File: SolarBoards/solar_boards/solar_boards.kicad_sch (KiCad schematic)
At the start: 18 parts, among them J1 M55-6001242R, U1 TPS61089

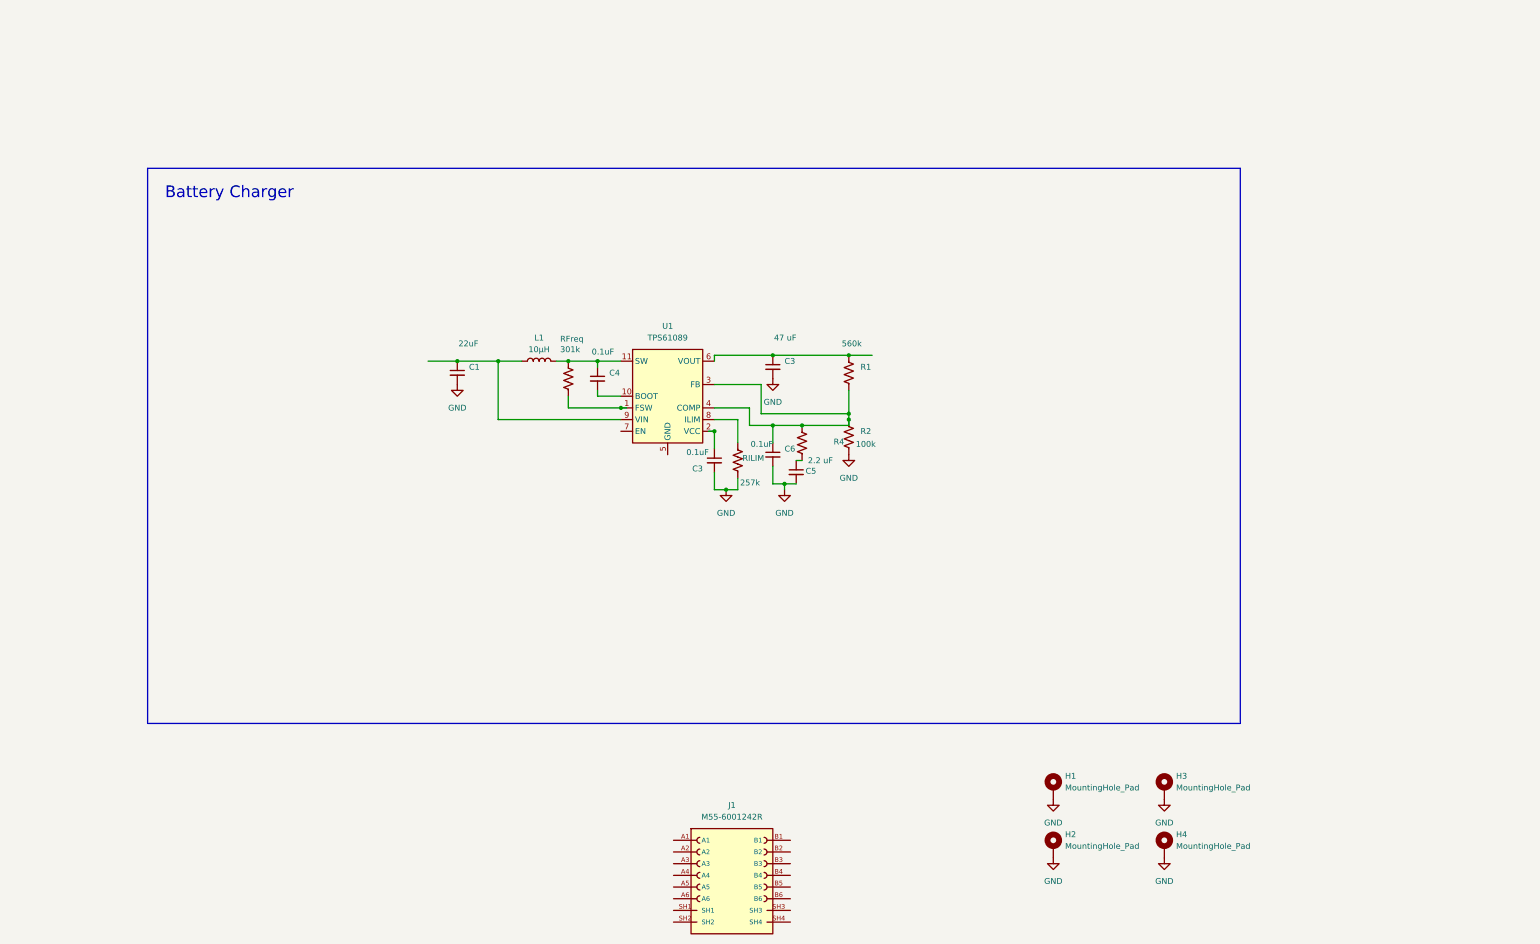
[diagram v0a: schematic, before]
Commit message: Solar Board Schematic and Routing
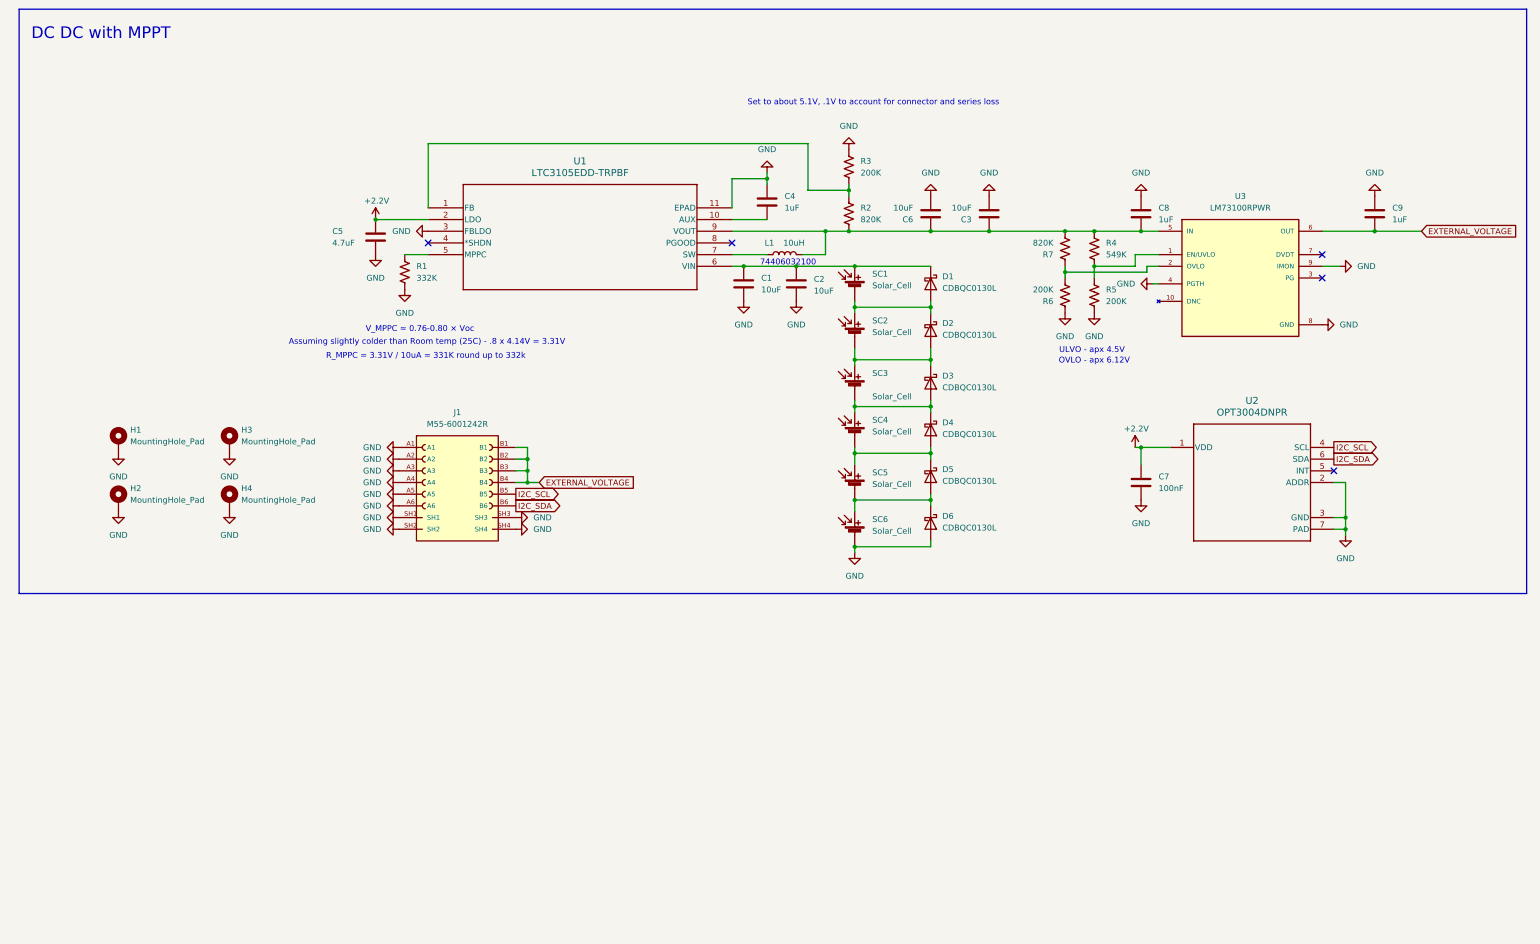
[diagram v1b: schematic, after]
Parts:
- removed C1: 22uF, symbol Device:C_Small
- removed C3: 47 uF, symbol Device:C_Small
- removed C3, C4, C6: 0.1uF, symbol Device:C_Small
- removed C5: 2.2 uF, symbol Device:C_Small
- removed RFreq: 301k, symbol Device:R_US
- removed RILIM: 257k, symbol Device:R_US
- removed U1: TPS61089, Package_DFN_QFN:Texas_VQFN-RNR0011A-11, symbol Regulator_Switching:TPS61089
- added C1, C2, C3, C6: 10uF, Capacitor_SMD:C_0402_1005Metric_Pad0.74x0.62mm_HandSolder, symbol Device:C
- added C4, C8, C9: 1uF, Capacitor_SMD:C_0402_1005Metric_Pad0.74x0.62mm_HandSolder, symbol Device:C
- added C5: 4.7uF, Capacitor_SMD:C_0402_1005Metric_Pad0.74x0.62mm_HandSolder, symbol Device:C
- added C7: 100nF, Capacitor_SMD:C_0402_1005Metric_Pad0.74x0.62mm_HandSolder, symbol Device:C
- added D1, D2, D3, D4, D5, D6: CDBQC0130L, inspireFly:DIODFN100X60X55-2N, symbol Device:D_Schottky
- added R3, R5, R6: 200K, Resistor_SMD:R_0402_1005Metric_Pad0.72x0.64mm_HandSolder, symbol Device:R_US
- added R7: 820K, Resistor_SMD:R_0402_1005Metric_Pad0.72x0.64mm_HandSolder, symbol Device:R_US
- added SC1, SC2, SC3, SC4, SC5, SC6: Solar_Cell, inspireFly:SOLAR_KXOB25-14X1F-TR, symbol Device:Solar_Cell
- added U1: LTC3105EDD-TRPBF, inspireFly:DFN-10_DD_LIT, symbol inspireFly:LTC3105EDD-TRPBF
- added U2: OPT3004DNPR, inspireFly:DNP0006A, symbol 2026-04-11_18-01-49:OPT3004DNPR
- added U3: LM73100RPWR, inspireFly:IC_LM73100RPWR, symbol inspireFly:LM73100RPWR
- L1: value 10µH -> 10uH; footprint (none) -> inspireFly:WE-LQFS_3818
- R1: value 560k -> 332K; footprint (none) -> Resistor_SMD:R_0402_1005Metric_Pad0.72x0.64mm_HandSolder
- R2: value 100k -> 820K; footprint (none) -> Resistor_SMD:R_0402_1005Metric_Pad0.72x0.64mm_HandSolder
- R4: value R_US -> 549K; footprint (none) -> Resistor_SMD:R_0402_1005Metric_Pad0.72x0.64mm_HandSolder
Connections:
- net GND: now also J1.A1, J1.A2, J1.A3, J1.A4, J1.A5, J1.A6, J1.SH1, J1.SH2, J1.SH3, J1.SH4, R1.2, C1.2, C2.2, C3.2, C4.1, C5.2, C6.2, C7.2, C8.2, C9.2, D6.2 (A), R3.1, R5.2, R6.1, SC6.2 (-), U1.11 (EPAD), U1.3 (FBLDO), U2.2 (ADDR), U2.3 (GND), U2.7 (PAD), U3.4 (PGTH), U3.8 (GND), U3.9 (IMON); no longer R2.2
- net at R4.2: now also R5.1, U3.1 (EN/UVLO)
- net at L1.1: now also U1.7 (SW)
- net at L1.2: now also R2.2, R4.1, C3.1, C6.1, C8.1, R7.2, U1.9 (VOUT), U3.5 (IN)
- net at R1.1: now also U1.5 (MPPC)
- net EXTERNAL_VOLTAGE: now reaches J1.B1
- net EXTERNAL_VOLTAGE: now also J1.B2, J1.B3, J1.B4, C9.1, U3.6 (OUT)
- net I2C_SCL: now reaches J1.B5
- net I2C_SCL: now also U2.4 (SCL)
- net I2C_SDA: now reaches J1.B6
- net I2C_SDA: now also U2.6 (SDA)
- new net: C1.1, C2.1, D1.1 (K), SC1.1 (+), U1.6 (VIN)
- new net: D1.2 (A), D2.1 (K), SC1.2 (-), SC2.1 (+)
- new net: D2.2 (A), D3.1 (K), SC2.2 (-), SC3.1 (+)
- new net: D4.2 (A), D5.1 (K), SC4.2 (-), SC5.1 (+)
- new net: D5.2 (A), D6.1 (K), SC5.2 (-), SC6.1 (+)
- new net: D3.2 (A), D4.1 (K), SC3.2 (-), SC4.1 (+)
- new net: R2.1, R3.2, U1.1 (FB)
- new net: C4.2, U1.10 (AUX)
- new net: R6.2, R7.1, U3.2 (OVLO)
- new net +2.2V: C5.1, C7.1, U1.2 (LDO), U2.1 (VDD)
- no-connect marks 0 -> 5
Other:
- note added: "74406032100"
- note added: "Assuming slightly colder than Room temp (25C) - .8 x 4.14V = 3.31V"
- note added: "DC DC with MPPT"
- note added: "OVLO - apx 6.12V"
- note added: "R_MPPC = 3.31V / 10uA = 331K round up to 332k"
- note added: "Set to about 5.1V, .1V to account for connector and series loss"
- note added: "ULVO - apx 4.5V"
- note added: "V_MPPC ≈ 0.76-0.80 × Voc"
- note removed: "Battery Charger"
- moved on the sheet: H1, H2, H3, H4, J1
